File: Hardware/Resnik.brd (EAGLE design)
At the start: 64.8 x 100 mm, 207 parts, among them IC1 ATMEGA644M, J1 CONN_82.54_SCREW, J3 CONN_42.54_SCREW, J4 CONN_82.54_SCREW, Q1 DMG3404, Q2 DMG3404, Q3 FDN360P, Q4 FDN360P, Q5 FDN360P, Q6 DMG3404, Q7 2N7002, Q8 2N7002, U1 TLV61220DBV, U10 TPS22917DBV, U11 SN74AUP1G04YFP, U12 SN74AUP1G04YFP, U13 SN74AUP1G04YFP, U14 SN74AUP2G08DQE, U15 SN74AUP2G08DQE, U16 SN74AUP2G08DQE, U17 MIC2544MSOP, U18 MIC2544MSOP, U19 MIC2544MSOP, U2 TPS62822DLC, U20 MIC2544MSOP, U21 TPS22917DBV, U22 TPS22917DBV, U23 FT231X-Q, U24 SN74LVC1G3157DRL, U25 SN74AUP3G34DCU, U26 TXS0102DQM, U27 TXS0108RGY, U28 TXS0108RGY, U29 TXS0104RGY, U3 TPS61032RSA, U30 MCP4726A2SOT-23, U31 BME280, U32 ADS1115, U33 ADS1115, U34 INA211DCK, U35 INA210DCK, U37 TLV3691DCK, U38 TS5A21366RSE, U39 MIC94090C6, U40 SN74AHC1G86DCK, U41 MCP23018QFN, U5 BQ2980RUG, U6 TPS2105, U7 LTC4412S6, U8 TPL5111DDC, U9 TPS79733

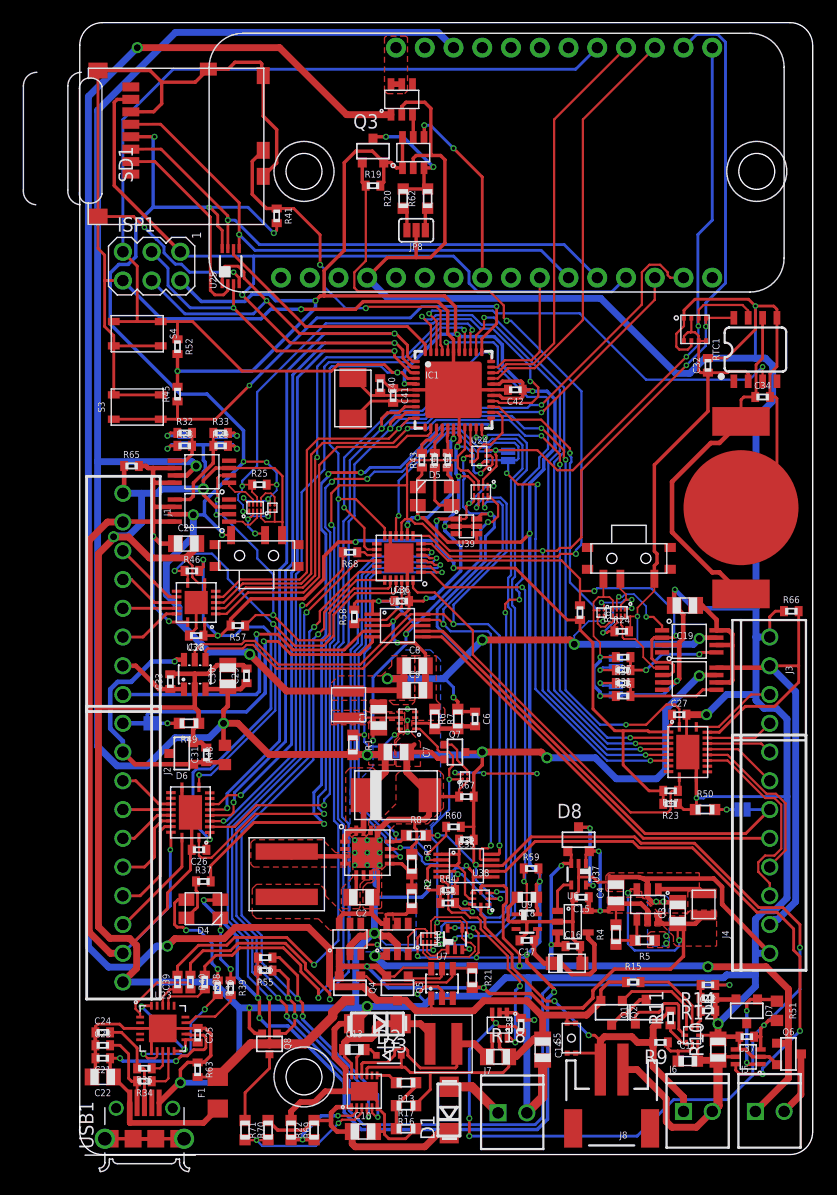
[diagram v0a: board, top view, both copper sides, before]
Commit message: Naming/part cleanup
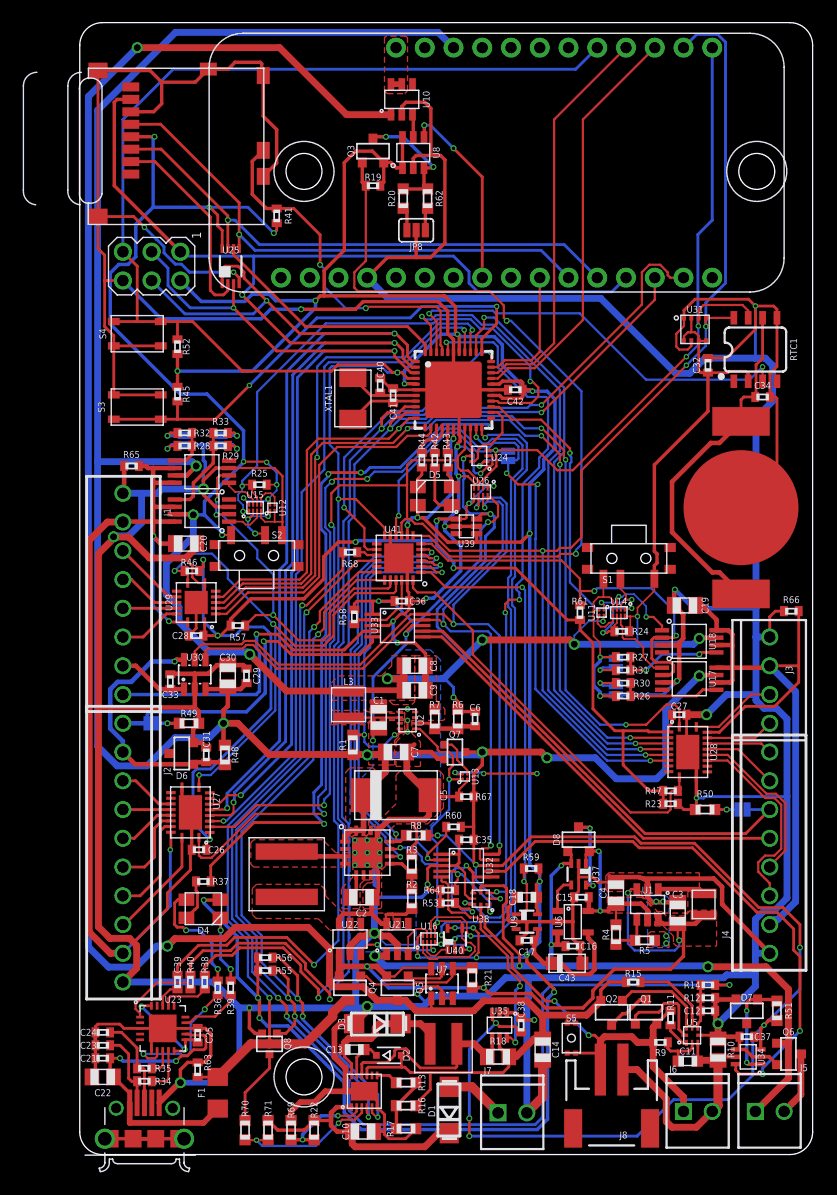
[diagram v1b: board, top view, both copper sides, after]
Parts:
- R12: value (none) -> 1k
- R22: value (none) -> 143k
- R51: value (none) -> 20k; device bschulz:R0603 -> bschulz_passives:R0603
- R55, R56, R59, R71: value (none) -> 1M
- R57, R58, R60, R61, R69: value (none) -> 100k
- R70: value (none) -> 200k
